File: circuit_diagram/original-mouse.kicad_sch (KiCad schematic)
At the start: 86 parts, among them J1 Conn_02x03_Odd_Even, J2 Conn_02x03_Odd_Even, Q1 TJ8S06M3L, Q10 ST-1KL3A, Q2 BSS138, Q3 BSS138, Q4 BSS138, Q5 BSS138, Q6 BSS138, Q7 ST-1KL3A, Q8 ST-1KL3A, Q9 ST-1KL3A, SW1 SW_SPDT, SW2 TS-06104, SW3 TS-06104, SW4 TS-06104, U1 NJM7805SDL1, U2 NJM2845DL1-33, U3 PKMCS0909E4000-R1, U4 ICM-20649, U5 DRV8835, U6 STM32F405RGTx

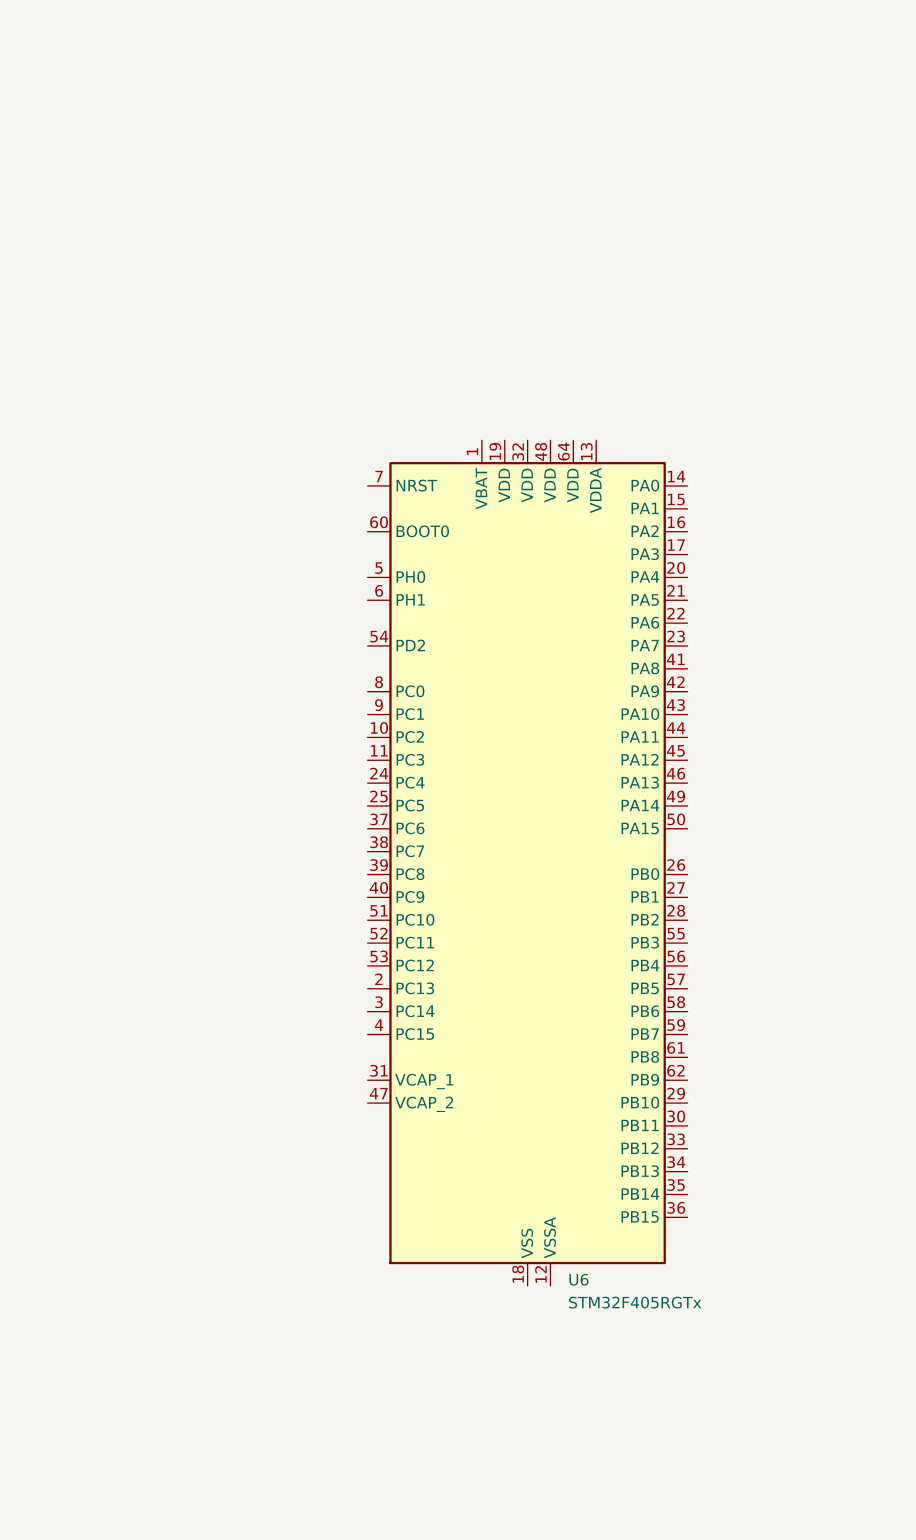
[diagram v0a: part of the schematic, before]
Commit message: update
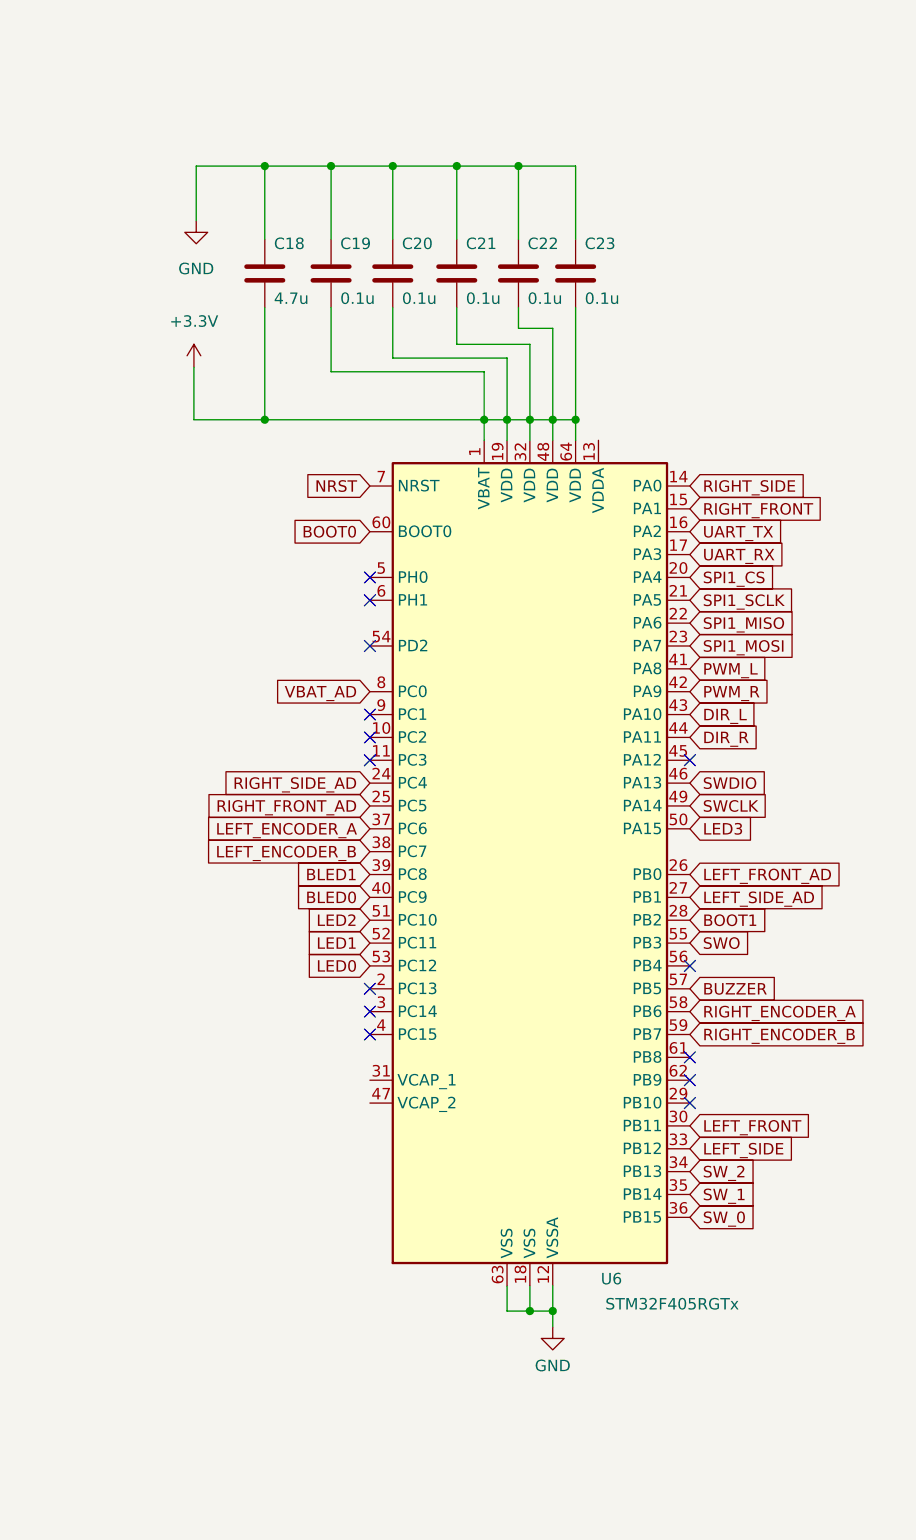
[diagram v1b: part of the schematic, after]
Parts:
- added C18: 4.7u, symbol Device:C
- added C19, C20, C21, C22, C23: 0.1u, symbol Device:C
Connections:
- net +3.3V: now also U6.1 (VBAT), U6.19 (VDD), U6.32 (VDD), U6.48 (VDD), U6.64 (VDD), C18.2, C19.2, C20.2, C21.2, C22.2, C23.2
- net BLED0: now also U6.40 (PC9)
- net BLED1: now also U6.39 (PC8)
- net DIR_L: now also U6.43 (PA10)
- net DIR_R: now also U6.44 (PA11)
- net GND: now also U6.12 (VSSA), U6.18 (VSS), U6.63 (VSS), C18.1, C19.1, C20.1, C21.1, C22.1, C23.1
- net LED0: now also U6.53 (PC12)
- net LED1: now also U6.52 (PC11)
- net LED2: now also U6.51 (PC10)
- net LED3: now also U6.50 (PA15)
- net LEFT_ENCODER_A: now also U6.37 (PC6)
- net LEFT_ENCODER_B: now also U6.38 (PC7)
- net LEFT_FRONT: now also U6.30 (PB11)
- net LEFT_FRONT_AD: now also U6.26 (PB0)
- net LEFT_SIDE: now also U6.33 (PB12)
- net LEFT_SIDE_AD: now also U6.27 (PB1)
- net PWM_L: now also U6.41 (PA8)
- net PWM_R: now also U6.42 (PA9)
- net RIGHT_ENCODER_A: now also U6.58 (PB6)
- net RIGHT_ENCODER_B: now also U6.59 (PB7)
- net RIGHT_FRONT: now also U6.15 (PA1)
- net RIGHT_FRONT_AD: now also U6.25 (PC5)
- net RIGHT_SIDE: now also U6.14 (PA0)
- net RIGHT_SIDE_AD: now also U6.24 (PC4)
- net SPI1_CS: now also U6.20 (PA4)
- net SPI1_MISO: now also U6.22 (PA6)
- net SPI1_MOSI: now also U6.23 (PA7)
- net SPI1_SCLK: now also U6.21 (PA5)
- net VBAT_AD: now also U6.8 (PC0)
- net UART_TX: now reaches U6.16 (PA2)
- net UART_RX: now reaches U6.17 (PA3)
- net BOOT1: now reaches U6.28 (PB2)
- net SW_2: now reaches U6.34 (PB13)
- net SW_1: now reaches U6.35 (PB14)
- net SW_0: now reaches U6.36 (PB15)
- net SWDIO: now reaches U6.46 (PA13)
- net SWCLK: now reaches U6.49 (PA14)
- net SWO: now reaches U6.55 (PB3)
- net BUZZER: now reaches U6.57 (PB5)
- net BOOT0: now reaches U6.60 (BOOT0)
- net NRST: now reaches U6.7 (NRST)
- no-connect marks 1 -> 15

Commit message: Update original-mouse.kicad_sch
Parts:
- added C24, C25: 2.2u, symbol Device:C
- added C26: 0.01u, symbol Device:C
- added C27, C29: 0.1u, symbol Device:C
- added C28: 1u, symbol Device:C
- added FB1: MZ1608-102Y, symbol Device:FerriteBead
- added J3: Conn_01x08, symbol Connector_Generic:Conn_01x08
- added R37: 10k, symbol Device:R
- added R38: R, symbol Device:R
- added SW5, SW6: SW_Push, symbol Switch:SW_Push
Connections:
- net Buzzer is gone; now on net BUZZER: RV1.3
- net SW_0 is gone; now on net SW0: U6.36 (PB15)
- net SW_1 is gone; now on net SW1: U6.35 (PB14)
- net SW_2 is gone; now on net SW2: U6.34 (PB13)
- net +3.3V: now also FB1.1, J3.1 (Pin_1), SW6.1
- net BOOT0: now also R38.1, SW6.2
- net GND: now also C24.2, C25.2, C26.2, C27.2, C28.2, C29.2, J3.3 (Pin_3), R37.2, R38.2, SW5.2
- net NRST: now also C29.1, J3.5 (Pin_5), SW5.1
- net SWCLK: now also J3.2 (Pin_2)
- net SWDIO: now also J3.4 (Pin_4)
- net SWO: now also J3.6 (Pin_6)
- net UART_RX: now also J3.7 (Pin_7)
- net UART_TX: now also J3.8 (Pin_8)
- net +3.3VA: now reaches U6.13 (VDDA)
- net +3.3VA: now also C26.1, C27.1, C28.1, FB1.2
- net at U6.31 (VCAP_1): now also C25.1
- net at U6.47 (VCAP_2): now also C24.1
- net +8V renamed +BATT
- net BOOT1: no longer names the net of U6.28 (PB2)
- net BOOT1: now also R37.1
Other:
- moved on the sheet: BT1, C1, C12, C13, C14, C15, C16, C17, C18, C19, C2, C20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
